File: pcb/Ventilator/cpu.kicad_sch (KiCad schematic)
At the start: 23 parts, among them J1 Conn_02x03_Top_Bottom, SW1 Reset, U1 W25Q128JVS, U2 RP2040

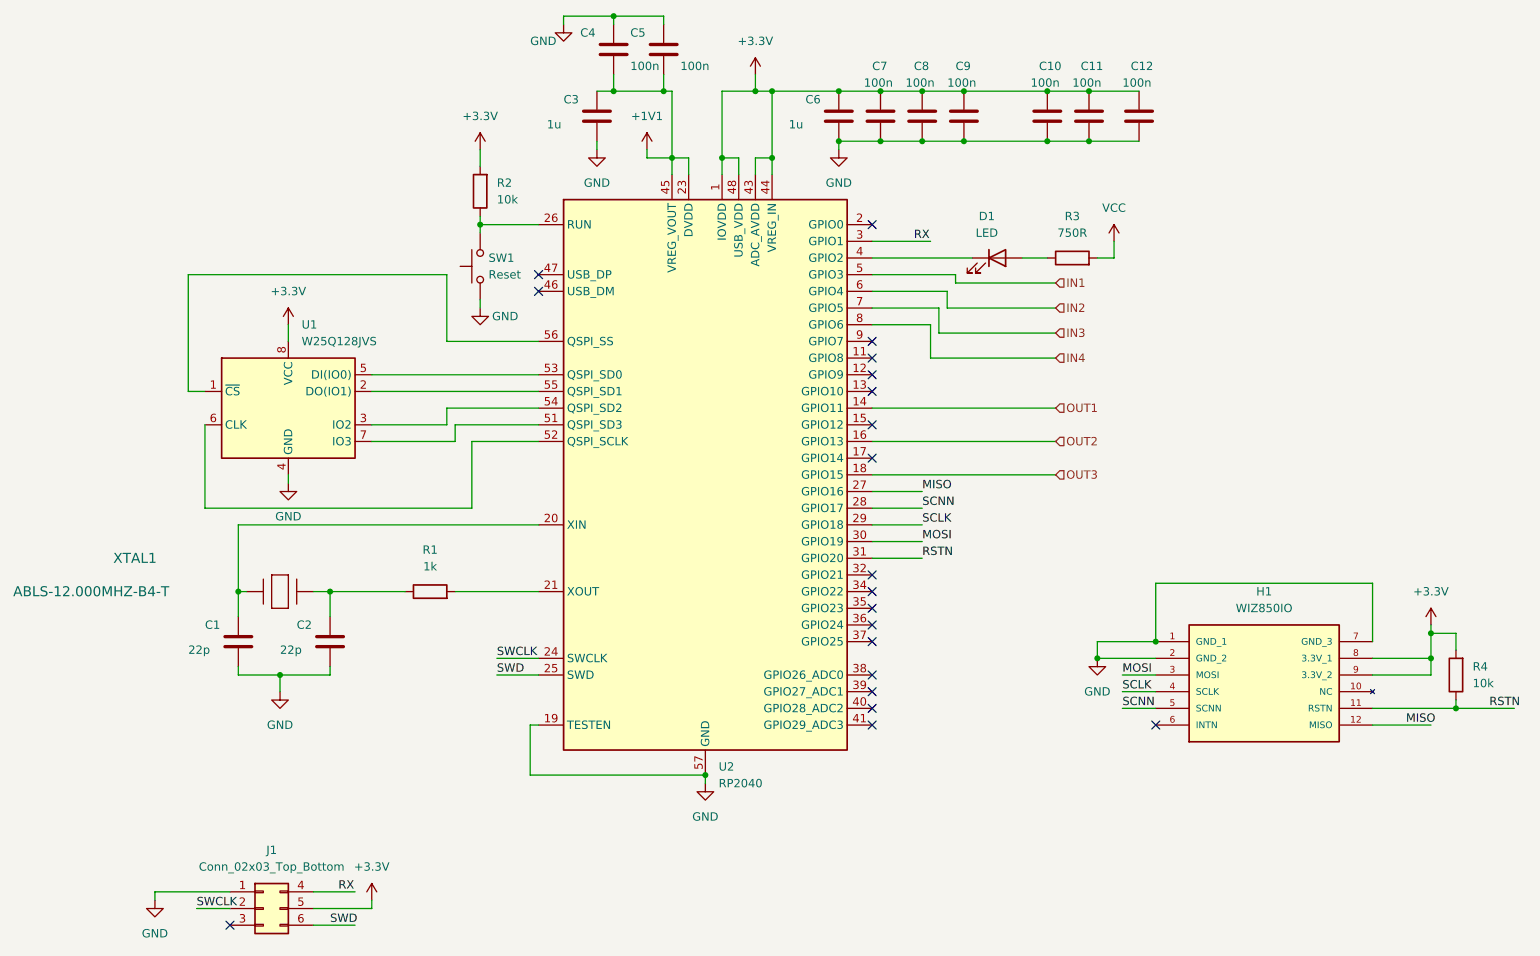
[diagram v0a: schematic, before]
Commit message: - voor autorouter
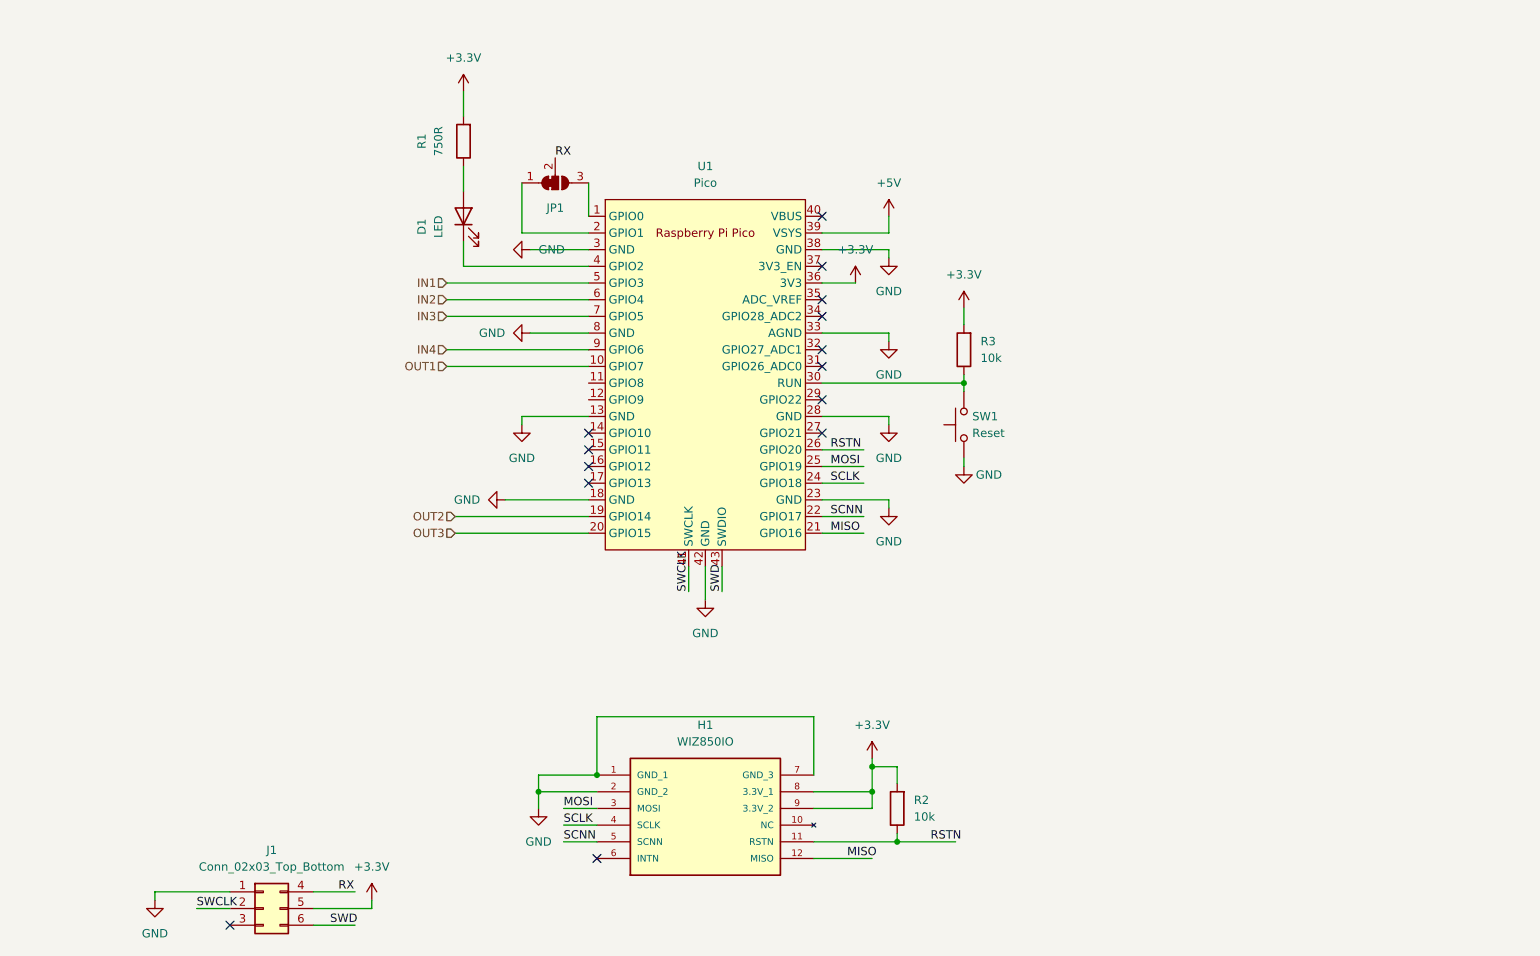
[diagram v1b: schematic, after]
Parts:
- removed C1, C2: 22p, Capacitor_SMD:C_1206_3216Metric_Pad1.33x1.80mm_HandSolder, symbol Device:C
- removed C10, C11, C12, C4, C5, C7, C8, C9: 100n, Capacitor_SMD:C_0805_2012Metric_Pad1.18x1.45mm_HandSolder, symbol Device:C
- removed C3, C6: 1u, Capacitor_SMD:C_0805_2012Metric_Pad1.18x1.45mm_HandSolder, symbol Device:C
- removed R1: 1k, Resistor_SMD:R_0805_2012Metric, symbol Device:R
- removed U1: W25Q128JVS, Package_SO:SOIC-8_5.23x5.23mm_P1.27mm, symbol Memory_Flash:W25Q128JVS
- removed U2: RP2040, Package_DFN_QFN:QFN-56-1EP_7x7mm_P0.4mm_EP3.2x3.2mm, symbol MCU_RaspberryPi:RP2040
- removed XTAL1: ABLS-12.000MHZ-B4-T, Xtal:ABLS-12.000MHZ-B4-T, symbol XTal:ABLS-12.000MHZ-B4-T
- added JP1: SolderJumper_3_Bridged12, Jumper:SolderJumper-3_P1.3mm_Bridged12_Pad1.0x1.5mm, symbol Jumper:SolderJumper_3_Bridged12
- added U1: Pico, MCU_RaspberryPi_and_Boards:RPi_Pico_SMD_TH, symbol MCU_RaspberryPi_and_Boards:Pico
- renumbered R3 to R1, R4 to R2, R2 to R3
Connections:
- net VCC is gone; now on net +3.3V: R1.2
- net +3.3V: now also U1.36 (3V3)
- net GND: now also U1.13 (GND), U1.18 (GND), U1.23 (GND), U1.28 (GND), U1.3 (GND), U1.33 (AGND), U1.38 (GND), U1.42 (GND), U1.8 (GND)
- net IN1: now also U1.5 (GPIO3)
- net IN2: now also U1.6 (GPIO4)
- net IN3: now also U1.7 (GPIO5)
- net IN4: now also U1.9 (GPIO6)
- net MISO: now also U1.21 (GPIO16)
- net MOSI: now also U1.25 (GPIO19)
- net OUT1: now also U1.10 (GPIO7)
- net OUT2: now also U1.19 (GPIO14)
- net OUT3: now also U1.20 (GPIO15)
- net RSTN: now also U1.26 (GPIO20)
- net RX: now also JP1.2 (C)
- net SCLK: now also U1.24 (GPIO18)
- net SCNN: now also U1.22 (GPIO17)
- net SWCLK: now also U1.41 (SWCLK)
- net SWD: now also U1.43 (SWDIO)
- net at R3.1, SW1.2: now also U1.30 (RUN)
- net at D1.1 (K): now also U1.4 (GPIO2)
- new net: JP1.1 (A), U1.2 (GPIO1)
- new net: JP1.3 (B), U1.1 (GPIO0)
- new net +5V: U1.39 (VSYS)
- no-connect marks 20 -> 14
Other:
- moved on the sheet: D1, H1, R1, R2, R3, SW1
